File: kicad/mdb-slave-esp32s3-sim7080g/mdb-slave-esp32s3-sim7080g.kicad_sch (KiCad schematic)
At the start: 81 parts, among them J1 USB_C_Receptacle_USB2.0_16P, J2 JAE_SIM_Card_SF72S006, J3 Conn_01x03_Pin, J4 Conn_Coaxial, J5 Conn_Coaxial, J6 MDB_Connector, J7 Conn_01x03_Pin, J8 Conn_01x04_Pin, Q1 MMBT3904, Q2 MMBT3904, Q3 MMBT3904, Q4 MMBT3904, Q5 MMBT3904, Q6 MMBT3904, Q7 MMBT3904, SW1 SW_Push, U1 ESP32-S3FH4R2, U2 SIM7080G, U3 LM2594HVM-3.3, U4 TLP785, U5 TLP785, Y1 Crystal_GND24

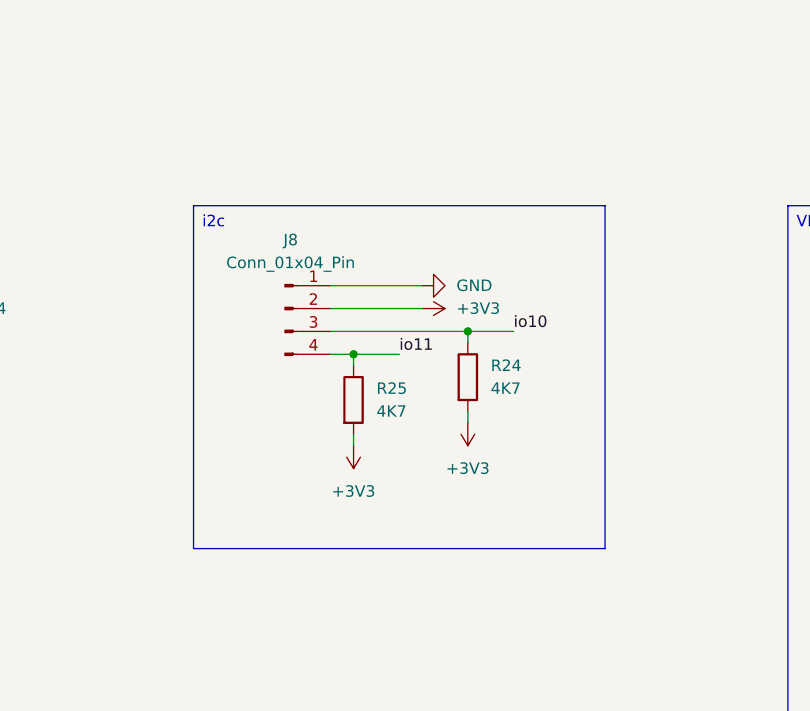
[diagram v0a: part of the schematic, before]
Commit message: chore(kicad): update schematic and PCB layouts
Co-Authored-By: Claude Opus 4.7 <noreply@anthropic.com>
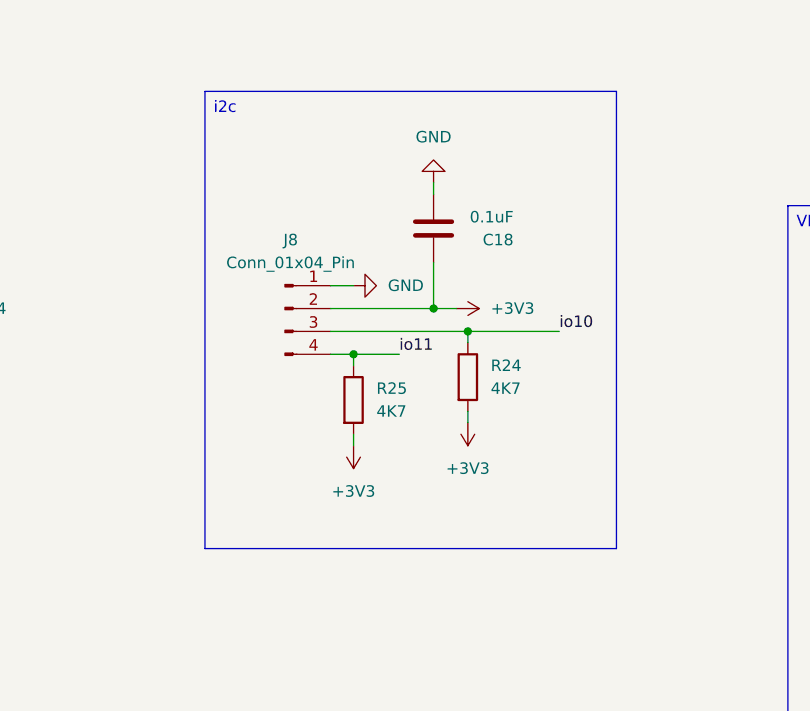
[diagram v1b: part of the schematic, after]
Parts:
- added C18: 0.1uF, Capacitor_SMD:C_0603_1608Metric, symbol Device:C
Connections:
- net +3V3: now also C18.1
- net GND: now also C18.2
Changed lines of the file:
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@@
 	(text_box "i2c"
 		(exclude_from_sim no)
-		(at 401.32 48.26 0)
-		(size 45.72 38.1)
+		(at 402.59 35.56 0)
+		(size 45.72 50.8)
 		(margins 0.9525 0.9525 0.9525 0.9525)
 		(stroke
@@
 	)
 	(junction
+		(at 427.99 59.69)
+		(diameter 0)
+		(color 0 0 0 0)
+	)
+	(junction
 		(at 259.08 270.51)
 		(diameter 0)
@@
 	(wire
 		(pts
-			(xy 416.56 59.69) (xy 426.72 59.69)
+			(xy 416.56 59.69) (xy 427.99 59.69)
 		)
 		(stroke
@@
 	(wire
 		(pts
+			(xy 427.99 45.72) (xy 427.99 46.99)
+		)
+		(stroke
+			(width 0)
+			(type default)
+		)
+	)
+	(wire
+		(pts
 			(xy 196.85 60.96) (xy 196.85 58.42)
 		)
@@
 	(wire
 		(pts
+			(xy 427.99 59.69) (xy 430.53 59.69)
+		)
+		(stroke
+			(width 0)
+			(type default)
+		)
+	)
+	(wire
+		(pts
 			(xy 165.1 148.59) (xy 167.64 148.59)
 		)
@@
 	(wire
 		(pts
-			(xy 426.72 57.15) (xy 416.56 57.15)
+			(xy 419.1 57.15) (xy 416.56 57.15)
 		)
 		(stroke
@@
 	(wire
 		(pts
-			(xy 431.8 62.23) (xy 436.88 62.23)
+			(xy 431.8 62.23) (xy 441.96 62.23)
 		)
 		(stroke
@@
 	(wire
 		(pts
+			(xy 427.99 54.61) (xy 427.99 59.69)
+		)
+		(stroke
+			(width 0)
+			(type default)
+		)
+	)
+	(wire
+		(pts
 			(xy 419.1 66.04) (xy 419.1 64.77)
 		)
@@
 	)
 	(label "io10"
-		(at 436.88 62.23 0)
+		(at 441.96 62.23 0)
 		(effects
 			(font
@@
 	)
 	(symbol
+		(lib_id "power:GND")
+		(at 427.99 45.72 180)
+		(unit 1)
+		(exclude_from_sim no)
+		(in_bom yes)
+		(on_board yes)
+		(dnp no)
+		(fields_autoplaced yes)
+		(property "Reference" "#PWR02"
+			(at 427.99 39.37 0)
+			(effects
+				(font
+					(size 1.27 1.27)
+				)
+				(hide yes)
+			)
+		)
+		(property "Value" "GND"
+			(at 427.99 40.64 0)
+			(effects
+				(font
+					(size 1.27 1.27)
+				)
+			)
+		)
+		(property "Footprint" ""
+			(at 427.99 45.72 0)
+			(effects
+				(font
+					(size 1.27 1.27)
+				)
+				(hide yes)
+			)
+		)
+		(property "Datasheet" ""
+			(at 427.99 45.72 0)
+			(effects
+				(font
+					(size 1.27 1.27)
+				)
+				(hide yes)
+			)
+		)
+		(property "Description" ""
+			(at 427.99 45.72 0)
+			(effects
+				(font
+					(size 1.27 1.27)
+				)
+				(hide yes)
+			)
+		)
+		(pin "1"
+		)
+		(instances
+			(project "mdb-slave-esp32s3-sim7080g"
+				(path "/95980b25-0707-441d-ba83-7f6c6e1d1aaa"
+					(reference "#PWR02")
+					(unit 1)
+				)
+			)
+		)
+	)
+	(symbol
 		(lib_id "Device:C")
 		(at 420.37 294.64 180)
@@
 	(symbol
 		(lib_id "power:GND")
-		(at 426.72 57.15 90)
+		(at 419.1 57.15 90)
 		(unit 1)
 		(exclude_from_sim no)
@@
 		(fields_autoplaced yes)
 		(property "Reference" "#PWR022"
-			(at 433.07 57.15 0)
+			(at 425.45 57.15 0)
 			(effects
 				(font
@@
 		)
 		(property "Value" "GND"
-			(at 430.53 57.1499 90)
+			(at 422.91 57.1499 90)
 			(effects
 				(font
@@
 		)
 		(property "Footprint" ""
-			(at 426.72 57.15 0)
+			(at 419.1 57.15 0)
 			(effects
 				(font
@@
 		)
 		(property "Datasheet" ""
-			(at 426.72 57.15 0)
+			(at 419.1 57.15 0)
 			(effects
 				(font
@@
 		)
 		(property "Description" ""
-			(at 426.72 57.15 0)
+			(at 419.1 57.15 0)
 			(effects
 				(font
@@
 	)
 	(symbol
+		(lib_id "Device:C")
+		(at 427.99 50.8 180)
+		(unit 1)
+		(exclude_from_sim no)
+		(in_bom yes)
+		(on_board yes)
+		(dnp no)
+		(property "Reference" "C18"
+			(at 436.88 52.07 0)
+			(effects
+				(font
+					(size 1.27 1.27)
+				)
+				(justify left)
+			)
+		)
+		(property "Value" "0.1uF"
+			(at 436.88 49.53 0)
+			(effects
+				(font
+					(size 1.27 1.27)
+				)
+				(justify left)
+			)
+		)
+		(property "Footprint" "Capacitor_SMD:C_0603_1608Metric"
+			(at 427.0248 46.99 0)
+			(effects
+				(font
+					(size 1.27 1.27)
+				)
+				(hide yes)
+			)
+		)
+		(property "Datasheet" "~"
+			(at 427.99 50.8 0)
+			(effects
+				(font
+					(size 1.27 1.27)
+				)
+				(hide yes)
+			)
+		)
+		(property "Description" ""
+			(at 427.99 50.8 0)
+			(effects
+				(font
+					(size 1.27 1.27)
+				)
+				(hide yes)
+			)
+		)
+		(property "LCSC#" "C5137636"
+			(at 427.99 50.8 90)
+			(effects
+				(font
+					(size 1.27 1.27)
+				)
+				(hide yes)
+			)
+		)
+		(property "Sim.Device" ""
+			(at 427.99 50.8 90)
+			(effects
+				(font
+					(size 1.27 1.27)
+				)
+				(hide yes)
+			)
+		)
+		(property "Sim.Pins" ""
+			(at 427.99 50.8 90)
+			(effects
+				(font
+					(size 1.27 1.27)
+				)
+				(hide yes)
+			)
+		)
+		(property "Sim.Type" ""
+			(at 427.99 50.8 90)
+			(effects
+				(font
+					(size 1.27 1.27)
+				)
+				(hide yes)
+			)
+		)
+		(pin "1"
+		)
+		(pin "2"
+		)
+		(instances
+			(project "mdb-slave-esp32s3-sim7080g"
+				(path "/95980b25-0707-441d-ba83-7f6c6e1d1aaa"
+					(reference "C18")
+					(unit 1)
+				)
+			)
+		)
+	)
+	(symbol
 		(lib_id "power:GND")
 		(at 265.43 257.81 180)
@@
 	(symbol
 		(lib_id "power:+3V3")
-		(at 426.72 59.69 270)
+		(at 430.53 59.69 270)
 		(unit 1)
 		(exclude_from_sim no)
@@
 		(fields_autoplaced yes)
 		(property "Reference" "#PWR021"
-			(at 422.91 59.69 0)
+			(at 426.72 59.69 0)
 			(effects
 				(font
@@
 		)
 		(property "Value" "+3V3"
-			(at 430.53 59.6899 90)
+			(at 434.34 59.6899 90)
 			(effects
 				(font
@@
 		)
 		(property "Footprint" ""
-			(at 426.72 59.69 0)
+			(at 430.53 59.69 0)
 			(effects
 				(font
@@
 		)
 		(property "Datasheet" ""
-			(at 426.72 59.69 0)
+			(at 430.53 59.69 0)
 			(effects
 				(font
@@
 		)
 		(property "Description" ""
-			(at 426.72 59.69 0)
+			(at 430.53 59.69 0)
 			(effects
 				(font
